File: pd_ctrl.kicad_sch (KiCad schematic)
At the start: 11 parts, among them U12 PD70100ILD-TR

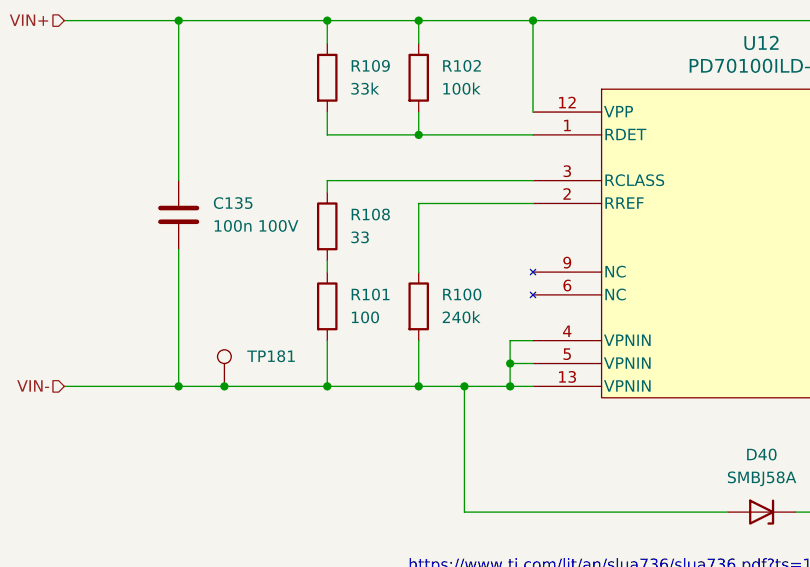
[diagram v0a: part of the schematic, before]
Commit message: fixed a lot of review comments
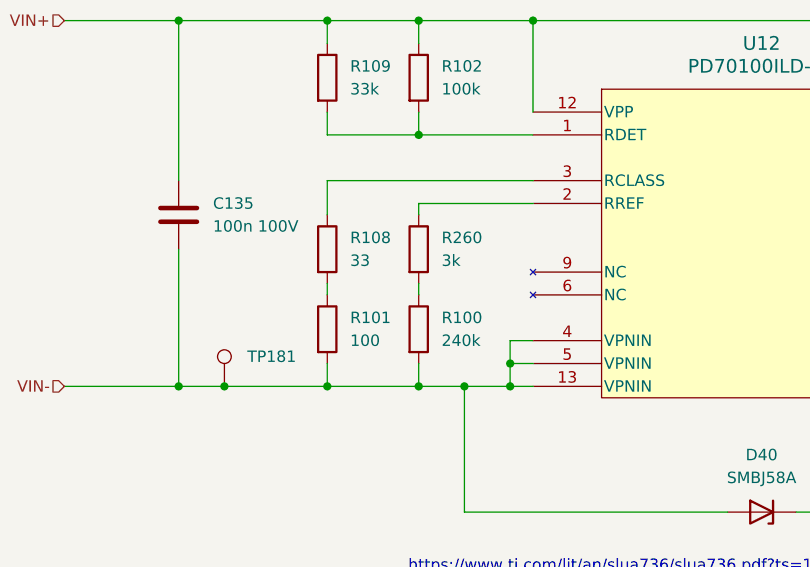
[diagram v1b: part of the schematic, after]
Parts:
- added R260: 3k, Resistor_SMD:R_0402_1005Metric, symbol Device:R
- R100, R101, R102, R108: Tolerance (none) -> 1%
- R109: LCSC Basic/Pref x -> y; Tolerance (none) -> 1%
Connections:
- net at R100.1: now also R260.2; no longer U12.2 (RREF)
- new net: R260.1, U12.2 (RREF)
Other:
- moved on the sheet: R100, R101, R108

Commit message: pre-changing properties
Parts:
- R101: LCSC Basic/Pref x -> y; LCSC missing (none) -> n; MPN (none) -> 0402WGF1000TCE; Manufacturer (none) -> UNI-ROYAL(Uniroyal Elec); Power (none) -> 62.5mW; Voltage (none) -> 50V
- R108: LCSC Basic/Pref x -> y; LCSC missing (none) -> n; MPN (none) -> 0402WGF330JTCE; Manufacturer (none) -> UNI-ROYAL; Power (none) -> 62.5mW; Voltage (none) -> 50V
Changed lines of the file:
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@@
 			)
 		)
-		(property "Datasheet" ""
+		(property "Datasheet" "https://www.lcsc.com/datasheet/C25105.pdf?spm=wm.sxq.inf.ggs&lcsc_vid=FFgPBABRR1JYAwZWRVhdVQZWEVcIBgBURANaBQVXQAUxVlNeT1dZUV1XTllbUzsOAxUeFF5JWBYZEEoKFBINSQcJGk4eFQsCAgIaSgADAwAHC0slRVRWUVNIHxUDCw%3D%3D"
 			(at 166.37 133.35 0)
 			(hide yes)
@@
 			)
 		)
-		(property "LCSC Basic/Pref" "x"
+		(property "LCSC Basic/Pref" "y"
 			(at 166.37 133.35 0)
 			(hide yes)
@@
 			)
 		)
-		(property "LCSC missing" ""
+		(property "LCSC missing" "n"
 			(at 166.37 133.35 0)
 			(hide yes)
@@
 		)
 		(property "Tolerance" "1%"
+			(at 166.37 133.35 0)
+			(hide yes)
+			(show_name no)
+			(do_not_autoplace no)
+			(effects
+				(font
+					(size 1.27 1.27)
+				)
+			)
+		)
+		(property "MPN" "0402WGF330JTCE"
+			(at 166.37 133.35 0)
+			(hide yes)
+			(show_name no)
+			(do_not_autoplace no)
+			(effects
+				(font
+					(size 1.27 1.27)
+				)
+			)
+		)
+		(property "Manufacturer" "UNI-ROYAL"
+			(at 166.37 133.35 0)
+			(hide yes)
+			(show_name no)
+			(do_not_autoplace no)
+			(effects
+				(font
+					(size 1.27 1.27)
+				)
+			)
+		)
+		(property "Power" "62.5mW "
+			(at 166.37 133.35 0)
+			(hide yes)
+			(show_name no)
+			(do_not_autoplace no)
+			(effects
+				(font
+					(size 1.27 1.27)
+				)
+			)
+		)
+		(property "Voltage" "50V"
 			(at 166.37 133.35 0)
 			(hide yes)
@@
 		)
 		(property "Tolerance" ""
+			(at 273.05 137.16 0)
+			(hide yes)
+			(show_name no)
+			(do_not_autoplace no)
+			(effects
+				(font
+					(size 1.27 1.27)
+				)
+			)
+		)
+		(property "Voltage" ""
 			(at 273.05 137.16 0)
 			(hide yes)
@@
 			)
 		)
+		(property "Voltage" ""
+			(at 154.94 148.59 0)
+			(hide yes)
+			(show_name no)
+			(do_not_autoplace no)
+			(effects
+				(font
+					(size 1.27 1.27)
+				)
+			)
+		)
 		(pin "1"
 		)
@@
 			)
 		)
+		(property "Voltage" ""
+			(at 214.63 162.56 0)
+			(hide yes)
+			(show_name no)
+			(do_not_autoplace no)
+			(effects
+				(font
+					(size 1.27 1.27)
+				)
+			)
+		)
 		(pin "2"
 		)
@@
 			)
 		)
+		(property "Voltage" ""
+			(at 176.53 142.24 0)
+			(hide yes)
+			(show_name no)
+			(do_not_autoplace no)
+			(effects
+				(font
+					(size 1.27 1.27)
+				)
+			)
+		)
 		(pin "1"
 		)
@@
 		)
 		(property "Tolerance" "1%"
+			(at 176.53 114.3 0)
+			(hide yes)
+			(show_name no)
+			(do_not_autoplace no)
+			(effects
+				(font
+					(size 1.27 1.27)
+				)
+			)
+		)
+		(property "Voltage" ""
 			(at 176.53 114.3 0)
 			(hide yes)
@@
 			)
 		)
+		(property "Voltage" ""
+			(at 256.54 138.43 0)
+			(hide yes)
+			(show_name no)
+			(do_not_autoplace no)
+			(effects
+				(font
+					(size 1.27 1.27)
+				)
+			)
+		)
 		(pin "1"
 		)
@@
 			)
 		)
+		(property "Voltage" ""
+			(at 189.23 123.19 0)
+			(hide yes)
+			(show_name no)
+			(do_not_autoplace no)
+			(effects
+				(font
+					(size 1.27 1.27)
+				)
+			)
+		)
 		(pin "8"
 		)
@@
 			)
 		)
+		(property "Voltage" ""
+			(at 176.53 133.35 0)
+			(hide yes)
+			(show_name no)
+			(do_not_autoplace no)
+			(effects
+				(font
+					(size 1.27 1.27)
+				)
+			)
+		)
 		(pin "1"
 		)
@@
 			)
 		)
+		(property "Voltage" ""
+			(at 166.37 114.3 0)
+			(hide yes)
+			(show_name no)
+			(do_not_autoplace no)
+			(effects
+				(font
+					(size 1.27 1.27)
+				)
+			)
+		)
 		(pin "1"
 		)
@@
 			)
 		)
+		(property "Voltage" ""
+			(at 149.86 129.54 0)
+			(hide yes)
+			(show_name no)
+			(do_not_autoplace no)
+			(effects
+				(font
+					(size 1.27 1.27)
+				)
+			)
+		)
 		(pin "2"
 		)
@@
 			)
 		)
-		(property "Datasheet" ""
+		(property "Datasheet" "https://jlc-prod-smt.oss-eu-central-1.aliyuncs.com/smtDataManualFile/8579705907476807680-C25076.pdf?response-content-disposition=attachment%3B%20filename%3DC25076.pdf%3B%20filename%2A%3DUTF-8%27%27C25076.pdf&x-oss-date=20260906T075419Z&x-oss-expires=1800&x-oss-security-token=CAISgAN1q6Ft5B2yfSjIr5qMIo%2Fco%2Bl34aG7RlLVlmlsSc5et%2FHlujz2IHhMdHJsAOodtv0%2FmmhT6PkclqRLcbhpcmfjV%2BZHzLB8qZN0slIu557b16cNrbH4M4H6aXeirtuwDsz9SNTCALjPD3nPii50x5bjaDymRCbLGJaViJlhHLN1Ow6jdmhpCctxLAlvo9NgFxm3D%2Fu2NQPwiWf9FVdhvhEG6Vly8qOi2MaRmFy8yFTx0b0SvJ%2BjYMrmPctoN9JnSdC5mfdzau3a1TJ84gRD0a5wkaVA1zbDs5bfISEIuUzebreLqY03dV4mOvdqIcMe8qigz88fk%2FfIioH6xyxKOexoSCnFTOiiupCcQLPyao9jLu6iayqViY7QaIOTqQohZmkAMwVOasAsI3Ngh4zF97Qt0cVNkXO9gWfLI8DtuMleWgrMe4k2SPZqaIWzHOTEFupYY7CDV2HC3D82fcxJ2B%2Bmz7zwy%2B%2Fdqxot7SHZVvl3SE4LlO17v1wIU7UcxaKWD5sagAEeJF5oW6mSsCUe8S%2BPvghauFqBb2F7v0lsc%2Btd4t6iV5UqXD5aRdOZ8Wr136%2Bp9FE%2BtyDG98O285bxV2GMu9tmAGVukYy7%2FyEFnvS2tCeov1zfWJYn3F%2FbG7PCWZhAQt7oPRDmWPsfXqnJEGwNadl31Rm55%2B7vOCxsV3UsHirdHyAA&x-oss-signature-version=OSS4-HMAC-SHA256&x-oss-credential=STS.NY9i5hN6VVcPDtdri9EArX4NX%2F20260906%2Feu-central-1%2Foss%2Faliyun_v4_request&x-oss-signature=5bbe7e40bf58d6570109f1bf902fc8812ea380f28b0918994f9c3e2d2de21944"
 			(at 166.37 142.24 0)
 			(hide yes)
@@
 			)
 		)
-		(property "LCSC Basic/Pref" "x"
+		(property "LCSC Basic/Pref" "y"
 			(at 166.37 142.24 0)
 			(hide yes)
@@
 			)
 		)
-		(property "LCSC missing" ""
+		(property "LCSC missing" "n"
 			(at 166.37 142.24 0)
 			(hide yes)
@@
 			(at 166.37 142.24 0)
 			(hide yes)
+			(show_name no)
+			(do_not_autoplace no)
+			(effects
+				(font
+					(size 1.27 1.27)
+				)
+			)
+		)
+		(property "Voltage" " 50V"
+			(at 166.37 142.24 0)
+			(hide yes)
+			(show_name no)
+			(do_not_autoplace no)
+			(effects
+				(font
+					(size 1.27 1.27)
+				)
+			)
+		)
+		(property "MPN" "0402WGF1000TCE"
+			(at 166.37 142.24 0)
+			(hide yes)
+			(show_name no)
+			(do_not_autoplace no)
+			(effects
+				(font
+					(size 1.27 1.27)
+				)
+			)
+		)
+		(property "Manufacturer" "UNI-ROYAL(Uniroyal Elec)"
+			(at 166.37 142.24 0)
+			(hide yes)
+			(show_name no)
+			(do_not_autoplace no)
+			(effects
+				(font
+					(size 1.27 1.27)
+				)
+			)
+		)
+		(property "Power" " 62.5mW"
+			(at 166.37 142.24 0)
+			(hide yes)
